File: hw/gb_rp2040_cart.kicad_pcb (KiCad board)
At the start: 4 copper layers, 51.4 x 60.5 mm, 75 parts, among them J1 GameBoy_Cartridge, J2 USB_C_Receptacle_USB2.0, Q1 SI2301CDS-T1-GE3, Q2 N-Channel, SW1 SW_DPST, SW2 SW_Push, U1 SN74LVC8T245PW, U10 MB85RC256VPNF-G-JNERE1, U11 DS3231M, U2 SN74LVC8T245PW, U3 TXU0104, U4 SN74LVC8T245PW, U5 W25Q128JVSIQ, U6 RP2040, U7 XC6206P332MR, U9 PCA9536D, Y1 Crystal_GND24

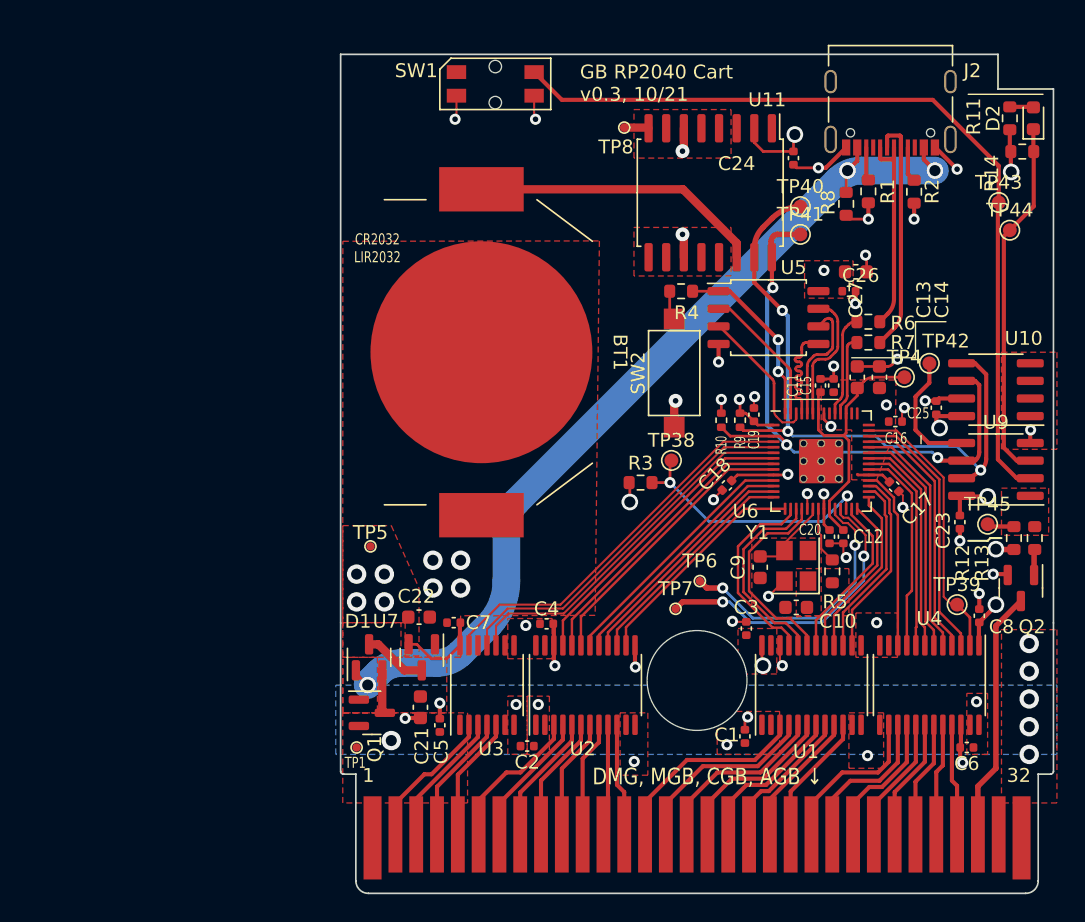
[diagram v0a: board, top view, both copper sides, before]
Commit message: hw: begin layout
Signed-off-by: Mahyar Koshkouei <mk@deltabeard.com>
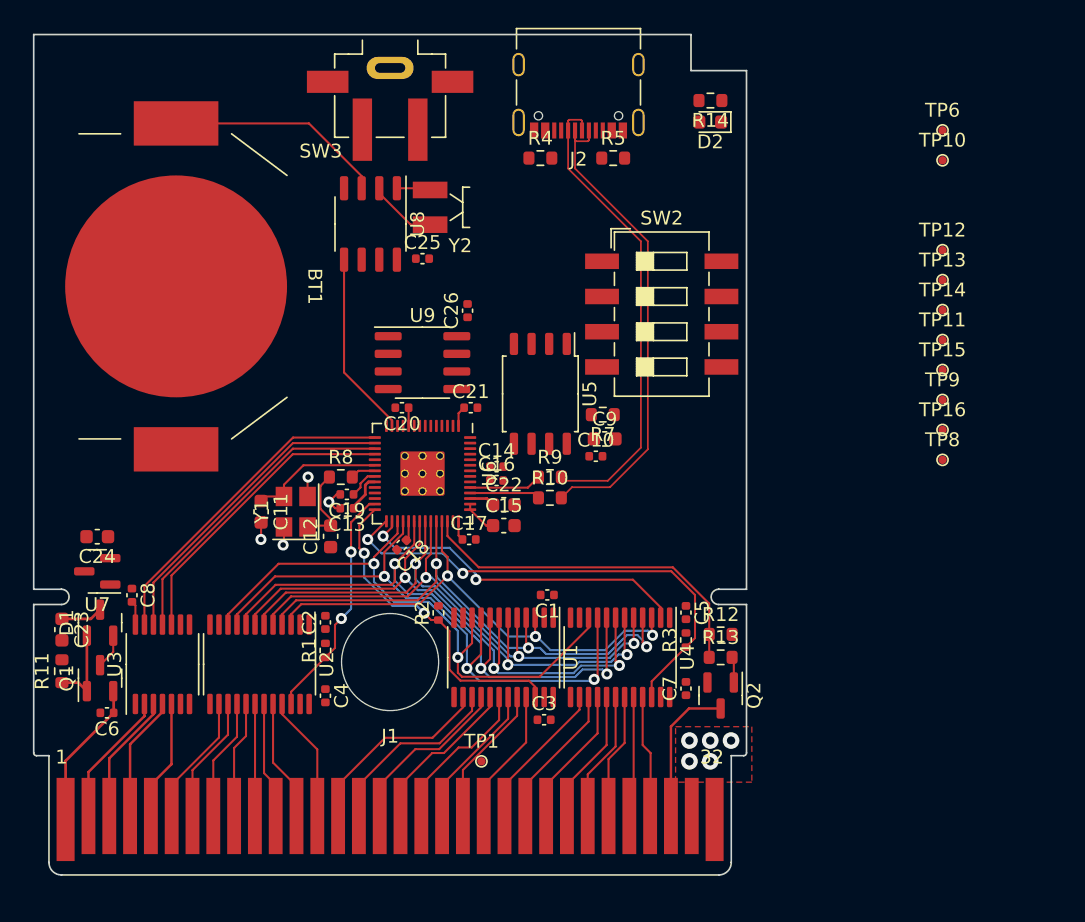
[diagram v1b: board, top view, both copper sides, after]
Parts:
- removed C27: 1u, Capacitor_SMD:C_0603_1608Metric
- removed R6: 27.4R, Resistor_SMD:R_0603_1608Metric
- removed SW1: SW_DPST, Project_Specific:K2-1114SA-A4SW-06
- removed TP38, TP39, TP40, TP41, TP42, TP43, TP44, TP45: TestPoint_Small, TestPoint:TestPoint_Pad_D1.0mm
- removed TP4, TP5: TestPoint, TestPoint:TestPoint_Pad_D1.0mm
- removed TP7: SWDIO, TestPoint:TestPoint_Pad_D1.0mm
- removed U10: MB85RC256VPNF-G-JNERE1, Package_SO:SOIC-8_3.9x4.9mm_P1.27mm
- removed U11: DS3231M, Package_SO:SOIC-16W_7.5x10.3mm_P1.27mm
- added SW3: SW_SPST, Project_Specific:TS-1037-A10B3-D2, F.Cu at (61.9, 39.5)
- added TP10: SWCLK, TestPoint:TestPoint_Pad_D1.0mm, F.Cu at (101.8, 45.2)
- added TP11: SWDIO, TestPoint:TestPoint_Pad_D1.0mm, F.Cu at (101.8, 58.1)
- added TP12: GND, TestPoint:TestPoint_Pad_D1.0mm, F.Cu at (101.8, 51.6)
- added TP13: TestPoint_Small, TestPoint:TestPoint_Pad_D1.0mm, F.Cu at (101.8, 53.8)
- added TP14: TestPoint_Small, TestPoint:TestPoint_Pad_D1.0mm, F.Cu at (101.8, 56.0)
- added TP15: TestPoint_Small, TestPoint:TestPoint_Pad_D1.0mm, F.Cu at (101.8, 60.3)
- added TP16: TestPoint_Small, TestPoint:TestPoint_Pad_D1.0mm, F.Cu at (101.8, 64.6)
- added TP9: TestPoint, TestPoint:TestPoint_Pad_D1.0mm, F.Cu at (101.8, 62.4)
- added U8: DS1307Z+, Package_SO:SO-8_3.9x4.9mm_P1.27mm, F.Cu at (60.5, 49.8)
- added Y2: 32.768k-12.5pF, Project_Specific:Crystal_DS26_D2.0mm_L6.0mm_Horizontal_1EP_style1, F.Cu at (65.3, 49.5)
- C10: value 30p -> 100n; footprint Capacitor_SMD:C_0603_1608Metric -> Capacitor_SMD:C_0402_1005Metric
- C11, C12: value 100n -> 30p; footprint Capacitor_SMD:C_0402_1005Metric -> Capacitor_SMD:C_0603_1608Metric
- C13, C14, C21: value 1u -> 100n; footprint Capacitor_SMD:C_0603_1608Metric -> Capacitor_SMD:C_0402_1005Metric
- C15, C23, C24: value 100n -> 1u; footprint Capacitor_SMD:C_0402_1005Metric -> Capacitor_SMD:C_0603_1608Metric
- C9: value 30p -> 1u
- R1, R2: value 5k1 -> 25k; footprint Resistor_SMD:R_0603_1608Metric -> Resistor_SMD:R_0402_1005Metric
- R10, R9: value 4k7 -> 27.4R; footprint Resistor_SMD:R_0402_1005Metric -> Resistor_SMD:R_0603_1608Metric
- R11: value 330R -> 100k
- R14: value 100k -> 330R
- R3: value 100k -> 25k; footprint Resistor_SMD:R_0603_1608Metric -> Resistor_SMD:R_0402_1005Metric
- R4, R5: value 1k -> 5k1
- R7: value 27.4R -> 1k
- R8: value 100k -> 1k
- SW2: value SW_Push -> SW_DIP_x04; footprint Button_Switch_SMD:SW_SPST_CK_RS282G05A3 -> Button_Switch_SMD:SW_DIP_SPSTx04_Slide_6.7x11.72mm_W8.61mm_P2.54mm_LowProfile
- TP1: value TestPoint -> TestPoint_Small
- TP6: value SWCLK -> TestPoint
- TP8: value GND -> TestPoint
- U9: value PCA9536D -> MB85RS256B
- moved R11 79.1 mm to (38.2, 82.0)
- moved C23 65.2 mm to (38.2, 79.0)
- moved C6 62.1 mm to (41.5, 85.0)
- moved C8 61.1 mm to (43.3, 76.5)
- moved C24 57.1 mm to (40.8, 72.3), turned to 180 degrees
- moved R1 51.3 mm to (57.2, 80.5)
- moved R2 45.8 mm to (65.4, 77.8), turned to 90 degrees
- moved U9 42.1 mm to (64.2, 59.8), turned to 0 degrees
- moved R8 41.4 mm to (58.4, 68.0), turned to 0 degrees
- moved C11 41.4 mm to (52.6, 70.5), turned to -90 degrees
- moved C25 38.6 mm to (64.2, 52.2), turned to 0 degrees
- moved C13 38.0 mm to (58.8, 70.2), turned to 180 degrees
- moved C12 37.0 mm to (57.6, 72.3), turned to 90 degrees
- moved TP6 36.9 mm to (101.8, 43.0)
- moved Y1 36.3 mm to (55.1, 70.5)
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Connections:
- BT1 pad 1: Net-(BT1-Pad1) -> V_{BAT}
- C1 pad 1: GB_5V -> +3V3
- C10 pad 1: GND -> +3V3
- C10 pad 2: Net-(C10-Pad2) -> GND
- C11 pad 1: +1V1 -> Net-(C11-Pad1)
- C12 pad 1: +1V1 -> GND
- C12 pad 2: GND -> Net-(C12-Pad2)
- C14 pad 1: +3V3 -> +1V1
- C2 pad 1: GB_5V -> +3V3
- C21 pad 1: +5V -> +3V3
- C22 pad 1: +3V3 -> +1V1
- C23 pad 1: +3V3 -> +5V
- C3 pad 2: +3V3 -> GB_5V
- C4 pad 2: +3V3 -> GB_5V
- C5 pad 1: GB_5V -> GND
- C5 pad 2: GND -> +3V3
- C7 pad 1: GND -> GB_5V
- C7 pad 2: +3V3 -> GND
- C9 pad 1: Net-(C9-Pad1) -> +3V3
- D2 pad 1: /Peripherals/STAT_LED -> Net-(D2-Pad1)
- D2 pad 2: Net-(D2-Pad2) -> STAT_LED
- R1 pad 1: GND -> ADDR1_OE
- R1 pad 2: Net-(J2-PadB5) -> +3V3
- R10 pad 1: I^{2}C_{SCL} -> Net-(R10-Pad1)
- R10 pad 2: +3V3 -> USB_DN
- R11 pad 1: +3V3 -> VBUS
- R11 pad 2: Net-(D2-Pad2) -> GND
- R12 pad 1: /Peripherals/GB_RESET -> GB_RESET
- R13 pad 1: /Peripherals/GB_RESET -> GB_RESET
- R14 pad 1: /Peripherals/STAT_LED -> Net-(D2-Pad1)
- R14 pad 2: +3V3 -> GND
- R2 pad 1: Net-(J2-PadA5) -> ADDR2_OE
- R2 pad 2: GND -> +3V3
- R3 pad 1: /RP2040/RUN -> DATA_OE
- R4 pad 1: /RP2040/USB_BOOT -> GND
- R4 pad 2: /RP2040/QSPI_SS -> Net-(J2-PadB5)
- R5 pad 1: Net-(C10-Pad2) -> Net-(J2-PadA5)
- R5 pad 2: Net-(R5-Pad2) -> GND
- R7 pad 1: Net-(R7-Pad1) -> /RP2040/USB_BOOT
- R7 pad 2: USB_DN -> /RP2040/QSPI_SS
- R8 pad 1: VBUS -> Net-(C12-Pad2)
- R8 pad 2: GND -> Net-(R8-Pad2)
- R9 pad 1: I^{2}C_{SDA} -> Net-(R9-Pad1)
- R9 pad 2: +3V3 -> USB_DP
- SW2 pad 1: GND -> Net-(SW2-Pad1)
- SW2 pad 2: /RP2040/USB_BOOT -> Net-(SW2-Pad2)
- TP1 pad 1: GB_5V -> /A15
- TP6 pad 1: /RP2040/SWCLK -> GB_5V
- TP8 pad 1: GND -> +1V1
- U1 pad 1: GB_5V -> +3V3
- U1 pad 10: /A15 -> 3V3_M0
- U1 pad 14: 3V3_A15 -> /A8
- U1 pad 15: 3V3_A14 -> /A9
- U1 pad 16: 3V3_A13 -> /A10
- U1 pad 17: 3V3_A12 -> /A11
- U1 pad 18: 3V3_A11 -> /A12
- U1 pad 19: 3V3_A10 -> /A13
- U1 pad 2: GB_5V -> GND
- U1 pad 20: 3V3_A9 -> /A14
- U1 pad 21: 3V3_A8 -> /A15
- U1 pad 22: GND -> ADDR2_OE
- U1 pad 23: +3V3 -> GB_5V
- U1 pad 24: +3V3 -> GB_5V
- U1 pad 3: /A8 -> 3V3_M7
- U1 pad 4: /A9 -> 3V3_M6
- U1 pad 5: /A10 -> 3V3_M5
- U1 pad 6: /A11 -> 3V3_M4
- U1 pad 7: /A12 -> 3V3_M3
- U1 pad 8: /A13 -> 3V3_M2
- U1 pad 9: /A14 -> 3V3_M1
- U2 pad 1: GB_5V -> +3V3
- U2 pad 10: /A7 -> 3V3_M0
- U2 pad 14: 3V3_A7 -> /A0
- U2 pad 15: 3V3_A6 -> /A1
- U2 pad 16: 3V3_A5 -> /A2
- U2 pad 17: 3V3_A4 -> /A3
- U2 pad 18: 3V3_A3 -> /A4
- U2 pad 19: 3V3_A2 -> /A5
- U2 pad 2: GB_5V -> GND
- U2 pad 20: 3V3_A1 -> /A6
- U2 pad 21: 3V3_A0 -> /A7
- U2 pad 22: GND -> ADDR1_OE
- U2 pad 23: +3V3 -> GB_5V
- U2 pad 24: +3V3 -> GB_5V
- U2 pad 3: /A0 -> 3V3_M7
- U2 pad 4: /A1 -> 3V3_M6
- U2 pad 5: /A2 -> 3V3_M5
- U2 pad 6: /A3 -> 3V3_M4
- U2 pad 7: /A4 -> 3V3_M3
- U2 pad 8: /A5 -> 3V3_M2
- U2 pad 9: /A6 -> 3V3_M1
- U4 pad 10: 3V3_D0 -> 3V3_M0
- U4 pad 22: GND -> DATA_OE
- U4 pad 3: 3V3_D7 -> 3V3_M7
- U4 pad 4: 3V3_D6 -> 3V3_M6
- U4 pad 5: 3V3_D5 -> 3V3_M5
- U4 pad 6: 3V3_D4 -> 3V3_M4
- U4 pad 7: 3V3_D3 -> 3V3_M3
- U4 pad 8: 3V3_D2 -> 3V3_M2
- U4 pad 9: 3V3_D1 -> 3V3_M1
- U6 pad 11: 3V3_A3 -> unconnected-(U6-Pad11)
- U6 pad 12: 3V3_A4 -> SWITCH
- U6 pad 13: 3V3_A5 -> I2C_{SDA}
- U6 pad 14: 3V3_A6 -> I2C_{SCLK}
- U6 pad 15: 3V3_A7 -> PHI_3V3
- U6 pad 16: 3V3_A8 -> ~{WR}_3V3
- U6 pad 17: 3V3_A9 -> ~{RD}_3V3
- U6 pad 18: 3V3_A10 -> ~{CS}_3V3
- U6 pad 2: I^{2}C_{SDA} -> Net-(SW2-Pad1)
- U6 pad 20: Net-(C9-Pad1) -> Net-(C11-Pad1)
- U6 pad 21: Net-(R5-Pad2) -> Net-(R8-Pad2)
- U6 pad 26: /RP2040/RUN -> unconnected-(U6-Pad26)
- U6 pad 27: 3V3_A11 -> ADDR1_OE
- U6 pad 28: 3V3_A12 -> ADDR2_OE
- U6 pad 29: 3V3_A13 -> DATA_OE
- U6 pad 3: I^{2}C_{SCL} -> Net-(SW2-Pad2)
- U6 pad 30: 3V3_A14 -> DATA_DIR
- U6 pad 31: 3V3_A15 -> 3V3_M0
- U6 pad 32: 3V3_D0 -> 3V3_M1
- U6 pad 34: 3V3_D1 -> 3V3_M2
- U6 pad 35: 3V3_D2 -> 3V3_M3
- U6 pad 36: 3V3_D3 -> 3V3_M4
- U6 pad 37: 3V3_D4 -> 3V3_M5
- U6 pad 38: 3V3_D5 -> 3V3_M6
- U6 pad 39: 3V3_D6 -> 3V3_M7
- U6 pad 4: PHI_3V3 -> Net-(SW2-Pad3)
- U6 pad 40: 3V3_D7 -> GB_RESET
- U6 pad 41: DATA_DIR -> STAT_LED
- U6 pad 46: Net-(R7-Pad1) -> Net-(R10-Pad1)
- U6 pad 47: Net-(R6-Pad1) -> Net-(R9-Pad1)
- U6 pad 5: ~{RD}_3V3 -> unconnected-(U6-Pad5)
- U6 pad 6: ~{CS}_3V3 -> SPI0_{MISO}
- U6 pad 7: 3V3_A0 -> SPI0_{CSn}
- U6 pad 8: 3V3_A1 -> SPI0_{SCK}
- U6 pad 9: 3V3_A2 -> SPI0_{MOSI}
- U9 pad 1: /Peripherals/GB_RESET -> SPI0_{CSn}
- U9 pad 2: /Peripherals/SWITCH -> SPI0_{MISO}
- U9 pad 3: /Peripherals/STAT_LED -> +3V3
- U9 pad 5: Net-(TP42-Pad1) -> SPI0_{MOSI}
- U9 pad 6: I^{2}C_{SCL} -> SPI0_{SCK}
- U9 pad 7: I^{2}C_{SDA} -> +3V3
- Y1 pad 1: Net-(C10-Pad2) -> Net-(C12-Pad2)
- Y1 pad 3: Net-(C9-Pad1) -> Net-(C11-Pad1)
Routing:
- net VBUS: track 66.5 -> 6.05 mm, vias 3 -> 0
- net /Peripherals/SWITCH: track 60.4 -> 0.00 mm
- net GND: track 58.0 -> 6.03 mm, vias 47 -> 9
- net I^{2}C_{SDA}: track 47.7 -> 0.00 mm, vias 3 -> 0
- net 3V3_M2: track 0.00 -> 46.2 mm, vias 0 -> 3
- net 3V3_M1: track 0.00 -> 45.4 mm, vias 0 -> 3
- net I^{2}C_{SCL}: track 44.0 -> 0.00 mm, vias 3 -> 0
- net 3V3_M3: track 0.00 -> 43.8 mm, vias 0 -> 3
- net 3V3_M0: track 0.00 -> 43.4 mm, vias 0 -> 2
- net 3V3_M4: track 0.00 -> 43.0 mm, vias 0 -> 3
- net 3V3_M6: track 0.00 -> 41.1 mm, vias 0 -> 3
- net 3V3_M5: track 0.00 -> 39.6 mm, vias 0 -> 3
- net 3V3_M7: track 0.00 -> 37.7 mm, vias 0 -> 3
- net DATA_OE: track 0.00 -> 35.9 mm, vias 0 -> 2
- net +3V3: track 45.2 -> 12.2 mm, vias 20 -> 0
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- removed copper zone on F.Cu, net +3V3
- removed copper zone on In2.Cu, net +3V3
- removed copper zone on F.Cu, net +5V
- removed copper zone on F.Cu, net /Peripherals/GB_RESET
- removed copper zone on B.Cu, net GB_5V
- removed copper zone on F.Cu, net GB_5V
- removed copper zone on In1.Cu, net GND
- removed copper zone on F.Cu, net Net-(C10-Pad2)
- removed copper zone on F.Cu, net VBUS
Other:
- board size 51.4 x 60.5 mm -> 51.4 x 60.6 mm
- copper layers 4 -> 2
- board text removed: "CR2032 LIR2032"
- board text removed: "DMG, MGB, CGB, AGB ↓"
- board text removed: "Flash cart compatible with DMG, MGB, CGB, AGB. Unlicensed product. Uses RP2040 with 16MiB NOR, 32KiB FRAM, RTC, USB-C. Design: United Kingdom, Assembly: P.R. China Copyright © 2021 Mahyar Koshkouei; Not for resale."
- board text removed: "GB RP2040 Cart v0.3, 10/21"
- board text removed: "JLCJLCJLCJLC"
- board text removed: "git.io/JEM5x"
